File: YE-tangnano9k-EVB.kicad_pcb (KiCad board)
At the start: 2 copper layers, 95 x 72 mm, 23 parts, among them J1 Conn_01x24_Socket, J2 Conn_01x24_Socket, Q1 2SC1815, SW1 SW_SPDT, SW2 SW_Push, SW3 SW_Push, U1 Tang Nano 9K, U2 OSL40391-IRA

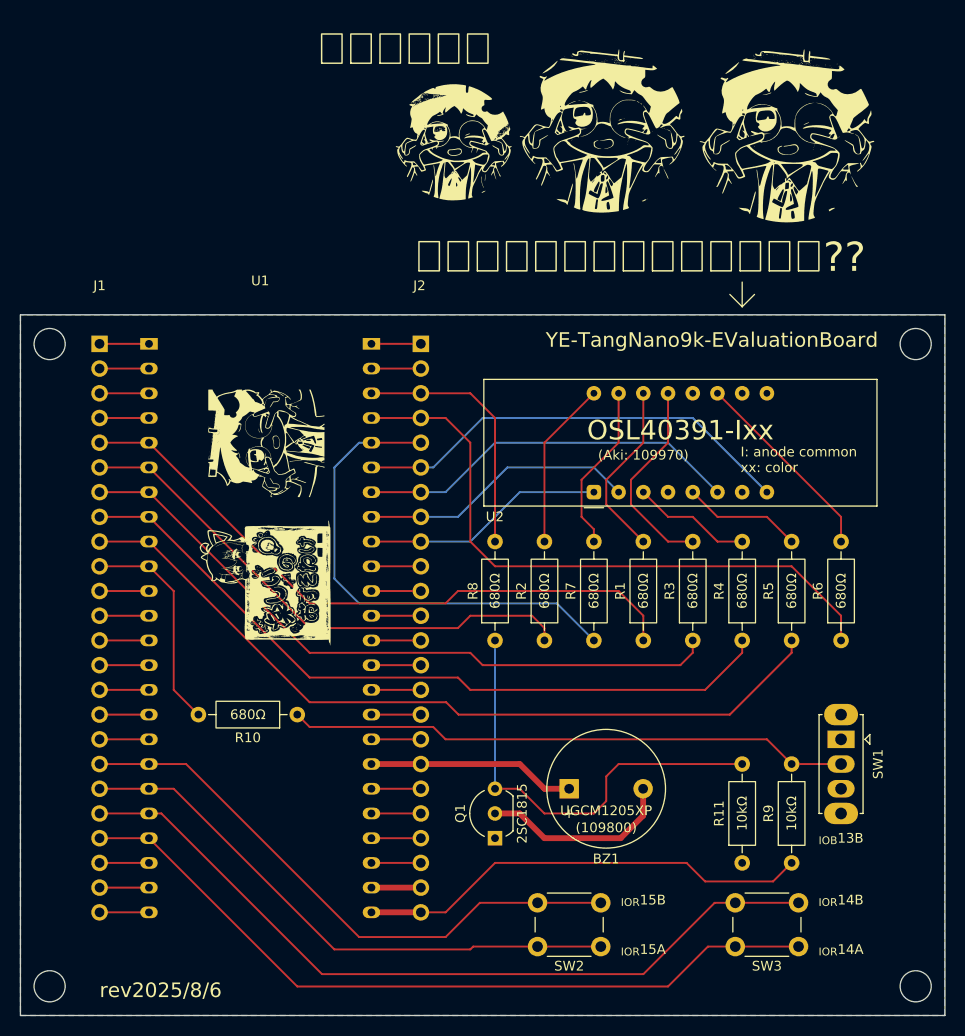
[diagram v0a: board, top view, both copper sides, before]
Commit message: 塗りつぶしをmeshに変更
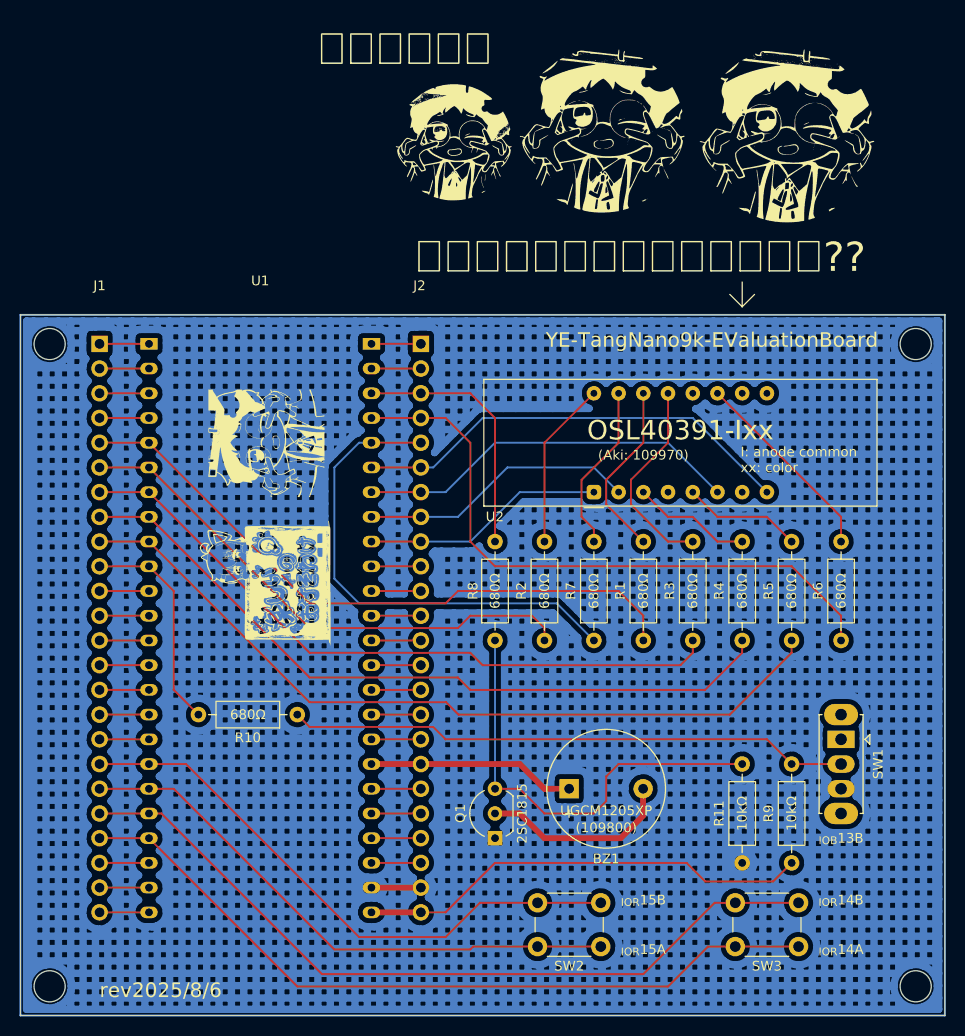
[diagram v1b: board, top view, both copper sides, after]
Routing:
- net GND: track 5.08 -> 9179.2 mm
- removed copper zone on B.Cu, net GND
